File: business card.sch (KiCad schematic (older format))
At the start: 9 parts

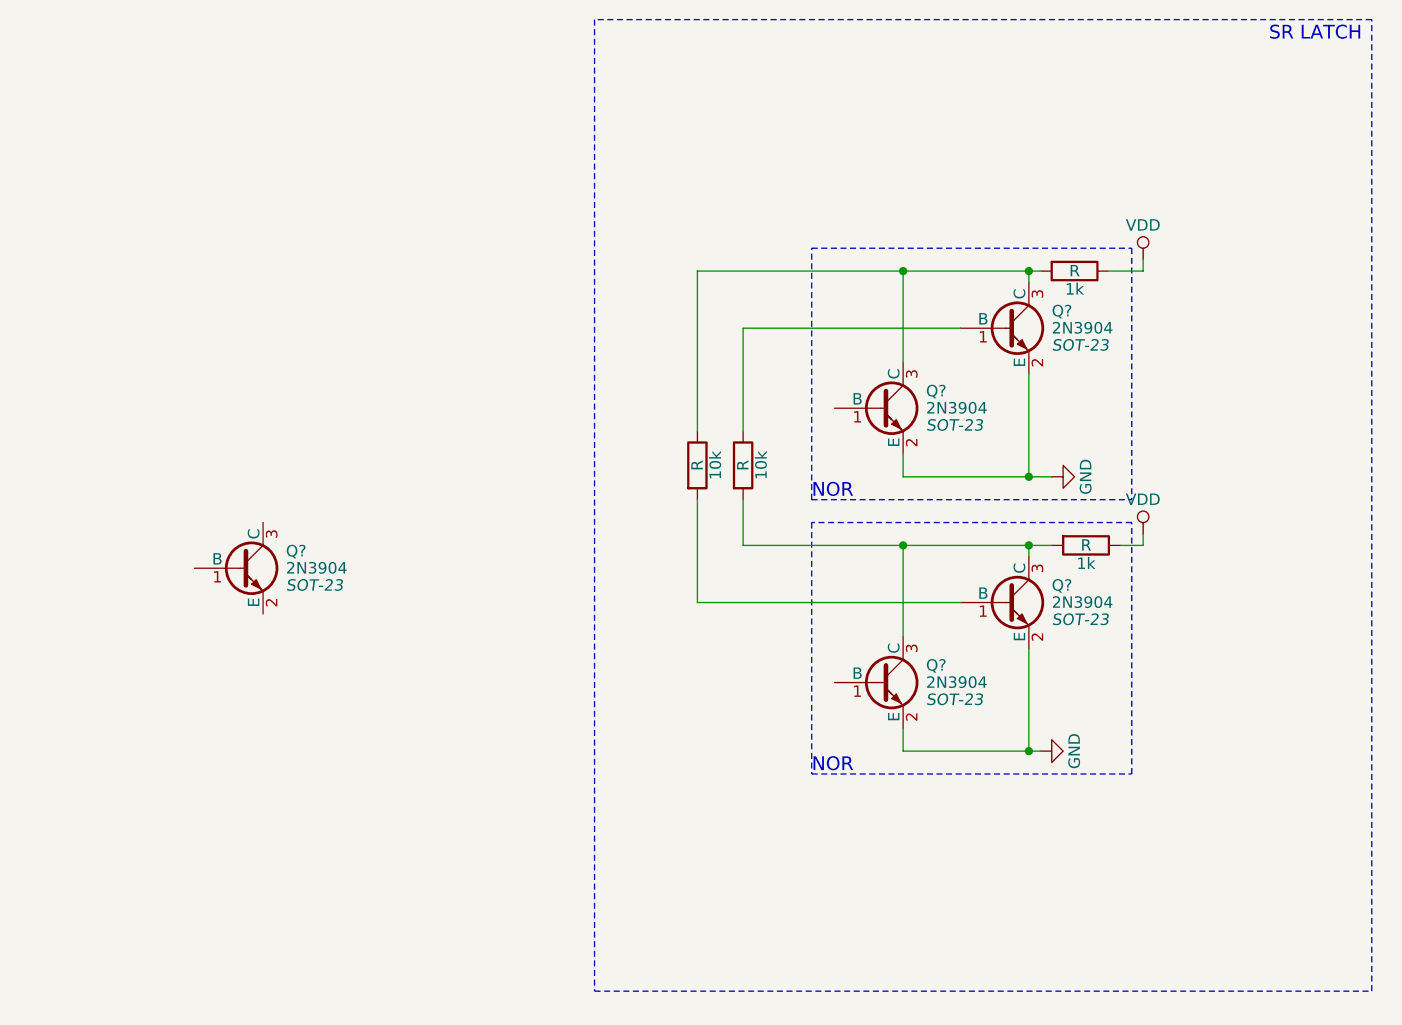
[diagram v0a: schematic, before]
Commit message: 17-6-10-2325
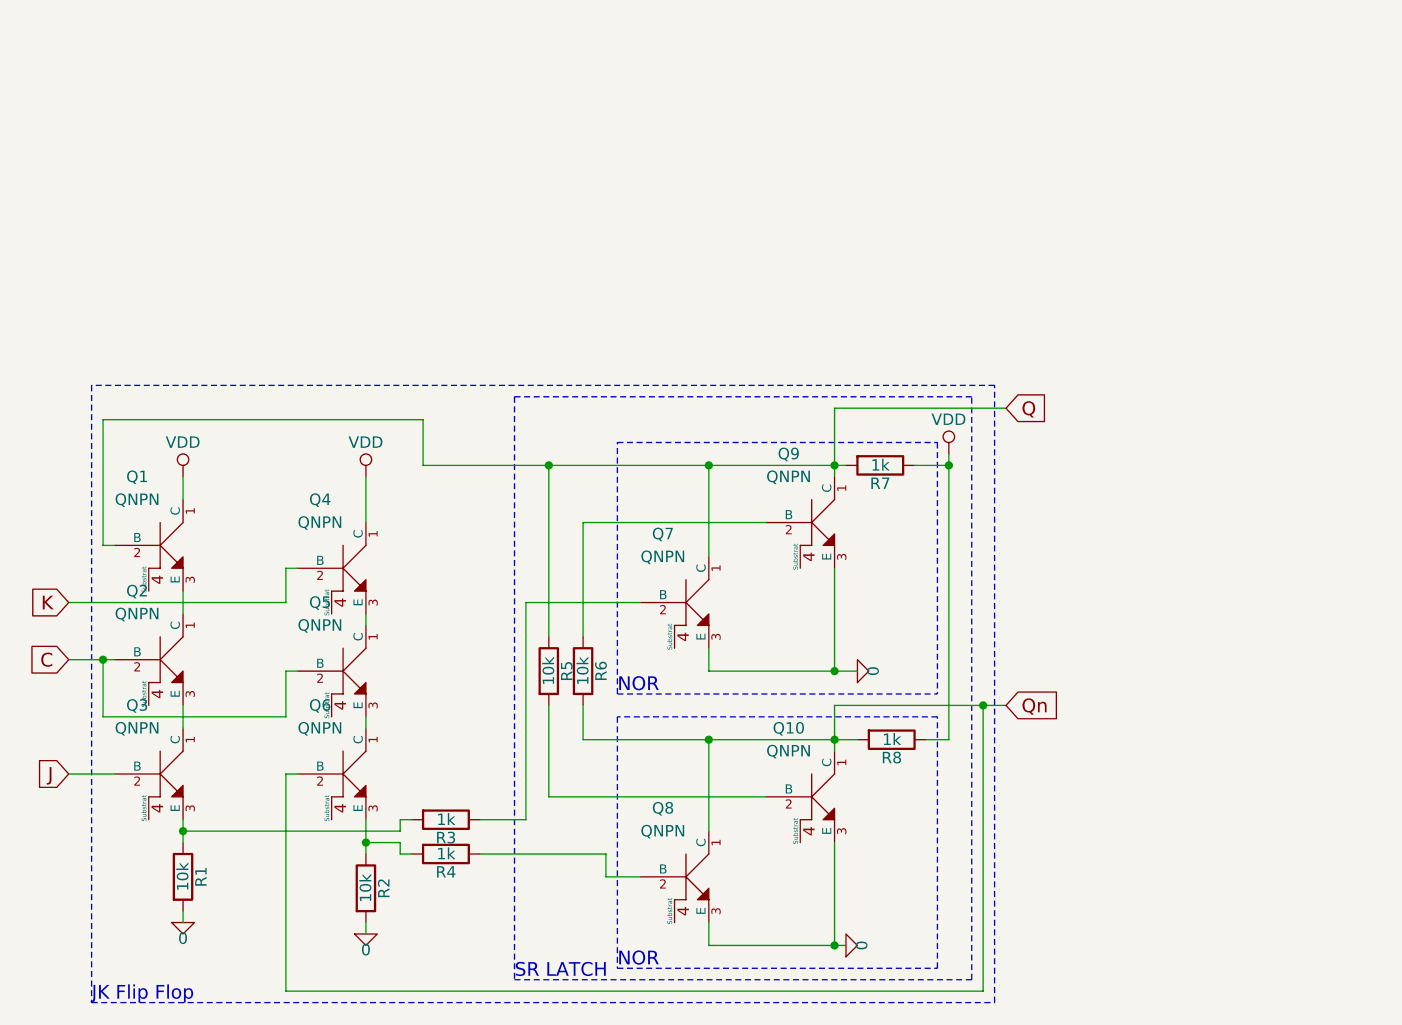
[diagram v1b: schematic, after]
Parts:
- removed 10k (x2), 1k (x2): R, symbol R
- removed Q? (x5): 2N3904, SOT-23, symbol 2N3904
- added Q1, Q10, Q2, Q3, Q4, Q5, Q6, Q7, Q8, Q9: QNPN, symbol QNPN
- added R1, R2, R5, R6: 10k, symbol R
- added R3, R4, R7, R8: 1k, symbol R
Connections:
- net VDD: now also Q1.1 (C), Q4.1 (C), R7.1, R8.1
- new net: Q1.3 (E), Q2.1 (C)
- new net: Q2.3 (E), Q3.1 (C)
- new net: Q3.3 (E), R1.1, R3.2
- new net: Q5.3 (E), Q6.1 (C)
- new net: Q6.3 (E), R2.1, R4.2
- new net: Q4.3 (E), Q5.1 (C)
- new net: Q9.2 (B), R6.1
- new net: Q7.2 (B), R3.1
- new net: Q8.2 (B), R4.1
- new net: Q10.2 (B), R5.2
- new net 0: Q10.3 (E), Q7.3 (E), Q8.3 (E), Q9.3 (E), R1.2, R2.2
- new net C: Q2.2 (B), Q5.2 (B)
- new net J: Q3.2 (B)
- new net K: Q4.2 (B)
- new net Q: Q1.2 (B), Q7.1 (C), Q9.1 (C), R5.1, R7.2
- new net Qn: Q10.1 (C), Q6.2 (B), Q8.1 (C), R6.2, R8.2
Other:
- note added: "JK Flip Flop\n"
